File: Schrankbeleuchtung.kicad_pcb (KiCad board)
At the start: 2 copper layers, 55 x 60 mm, 32 parts, among them J1 694106301002, J2 B2B-XH-AMLFSNP, J3 B2B-XH-AMLFSNP, J4 B2B-XH-AMLFSNP, J5 B2B-XH-AMLFSNP, J6 B2B-XH-AMLFSNP, J7 B2B-XH-AMLFSNP, J8 B2B-XH-AMLFSNP, J9 B2B-XH-AMLFSNP, Q1 IRLML6344, Q2 IRLML6344, Q3 IRLML6344, Q4 IRLML6344, U1 TPS560430XDBVT

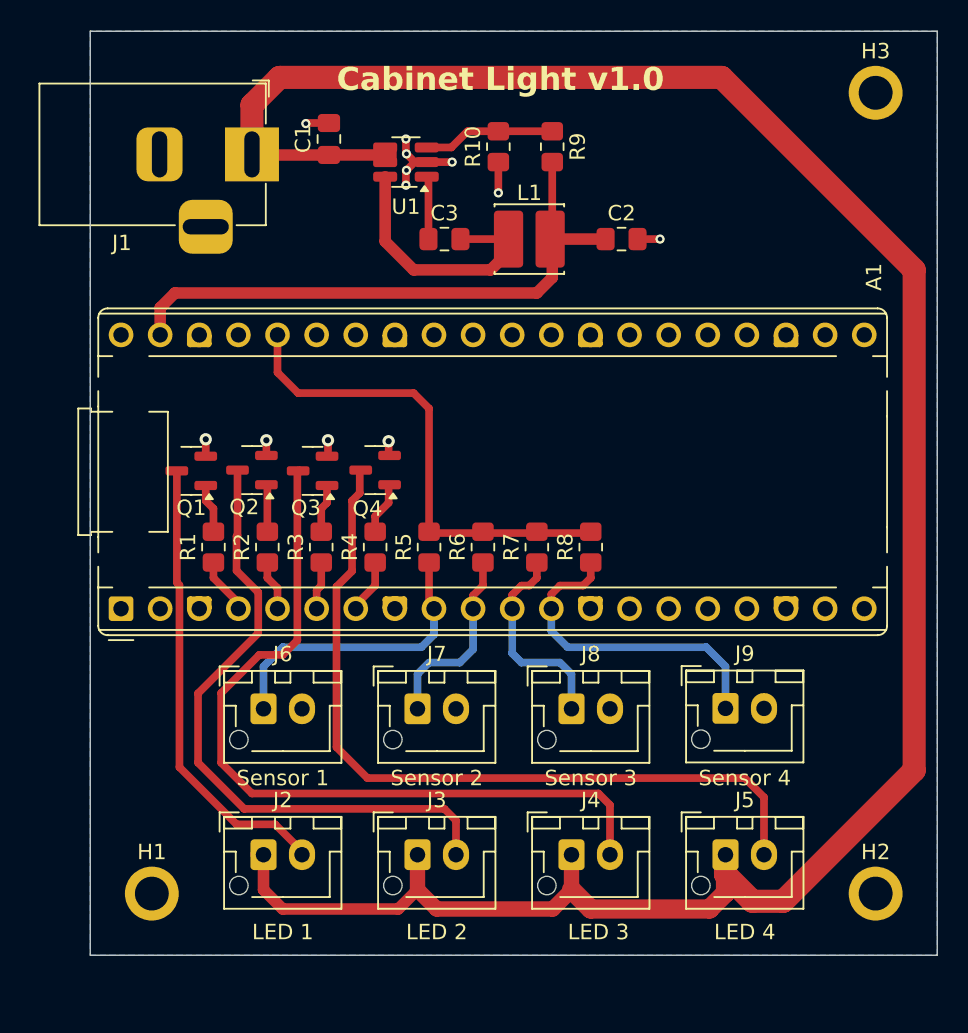
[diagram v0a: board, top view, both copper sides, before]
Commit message: PCB Layoutupdate
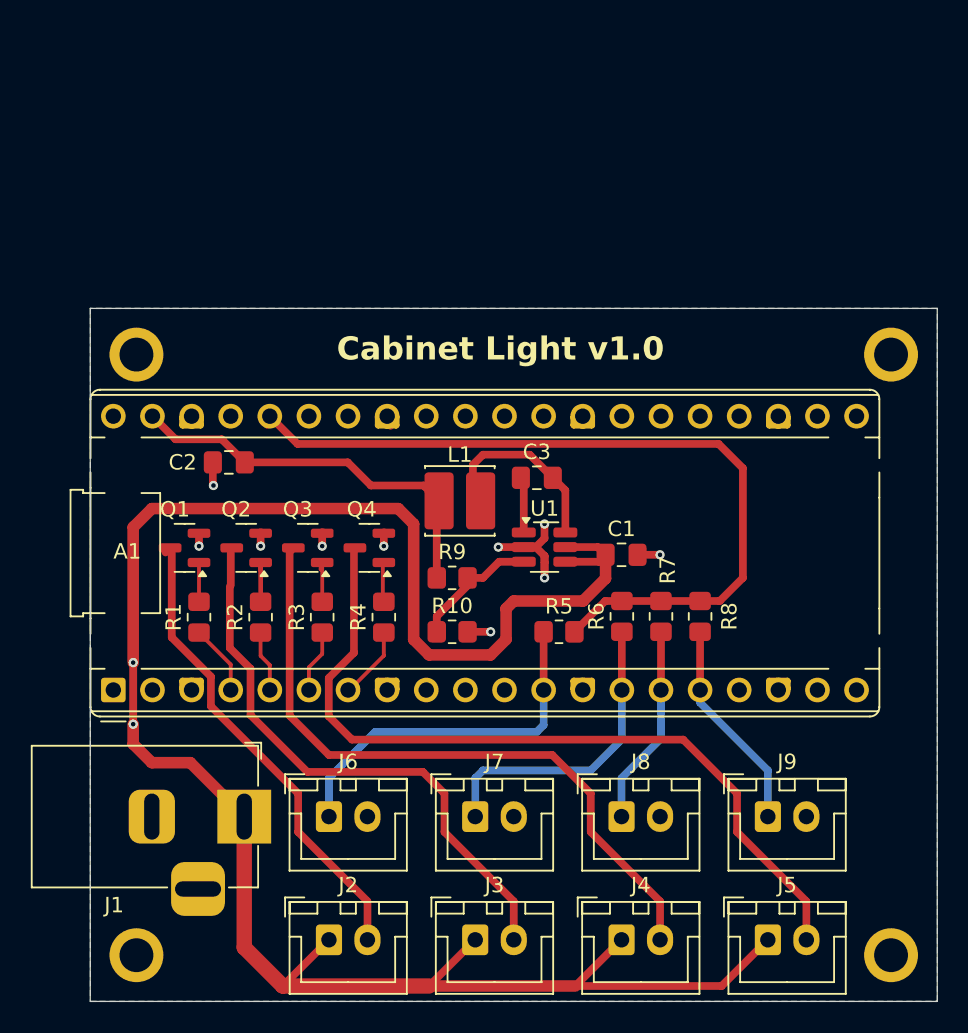
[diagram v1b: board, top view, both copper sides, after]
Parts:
- added H4: MountingHole_Pad, MountingHole:MountingHole_2.2mm_M2_ISO7380_Pad, F.Cu at (48.0, 48.0)
- J2, J3, J4, J5, J6, J7, J8, J9: footprint Connector_JST:JST_XH_B2B-XH-AM_1x02_P2.50mm_Vertical -> Connector_JST:JST_XH_B2B-XH-A_1x02_P2.50mm_Vertical
- Q1, Q2, Q3, Q4: value IRLML6344 -> IRLML0030TRPBF
- R1, R2, R3, R4: value 100R -> 187R
- moved J1 43.0 mm to (55.0, 78.0)
- moved C1 33.0 mm to (79.5, 61.0), turned to 0 degrees
- moved R10 31.6 mm to (68.5, 66.0), turned to 180 degrees
- moved C2 29.3 mm to (54.0, 55.0), turned to 180 degrees
- moved R9 28.7 mm to (68.5, 62.5), turned to 180 degrees
- moved U1 26.6 mm to (74.5, 60.5), turned to 0 degrees
- moved L1 17.6 mm to (69.0, 57.5), turned to 180 degrees
- moved H3 17.0 mm to (97.0, 48.0)
- moved C3 16.6 mm to (74.0, 56.0)
- moved R6 10.1 mm to (79.5, 65.0)
- moved R5 10.1 mm to (75.4, 66.0), turned to 0 degrees
- moved R7 9.23 mm to (82.1, 65.0)
- moved R8 8.41 mm to (84.6, 65.0)
- moved J6 8.19 mm to (60.5, 78.0)
- moved J7 7.94 mm to (70.0, 78.0)
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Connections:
- A1 pad 10: /GPIO07 -> unconnected-(A1-GPIO7-Pad10)
- A1 pad 11: /GPIO08 -> unconnected-(A1-GPIO8-Pad11)
- A1 pad 12: /GPIO09 -> /GPIO06
- A1 pad 14: unconnected-(A1-GPIO10-Pad14) -> /GPIO07
- A1 pad 15: unconnected-(A1-GPIO11-Pad15) -> /GPIO08
- A1 pad 16: unconnected-(A1-GPIO12-Pad16) -> /GPIO09
- A1 pad 9: /GPIO06 -> unconnected-(A1-GPIO6-Pad9)
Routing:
- net +12V: track 155.7 -> 134.7 mm, vias 0 -> 2
- net +3.3V: track 31.9 -> 51.7 mm
- net +5V: track 39.0 -> 26.0 mm
- net /GPIO09: track 21.8 -> 14.0 mm
- net /GPIO07: track 12.5 -> 20.2 mm
- net Net-(J4-Pin_2): track 51.6 -> 44.1 mm
- net Net-(U1-SW): track 17.2 -> 12.3 mm
- net Net-(J3-Pin_2): track 41.7 -> 37.4 mm
- net /GPIO06: track 19.9 -> 24.0 mm
- net Net-(Q2-G): track 3.11 -> 5.61 mm
- net /GPIO03: track 3.36 -> 4.98 mm
- net /GPIO04: track 3.21 -> 4.59 mm
- net /GPIO05: track 3.61 -> 4.94 mm
- net /GPIO02: track 3.76 -> 4.77 mm
- net Net-(J2-Pin_2): track 30.3 -> 31.2 mm
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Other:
- board size 55 x 60 mm -> 55 x 45 mm
